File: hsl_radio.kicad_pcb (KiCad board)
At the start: 4 copper layers, 95.9 x 90.2 mm, 77 parts, among them J2 CC Prog/Debug, J4 UART1, J5 Control Outputs, J6 ANT, U1 AP62300TWU-7, U10 SKY65366-21, U2 CC1110, U3 SF2446E, U4 PCI-104, U5 TLV803S, U6 PE4259, U7 0433BM15A0001, U8 FT5HN 27MHz

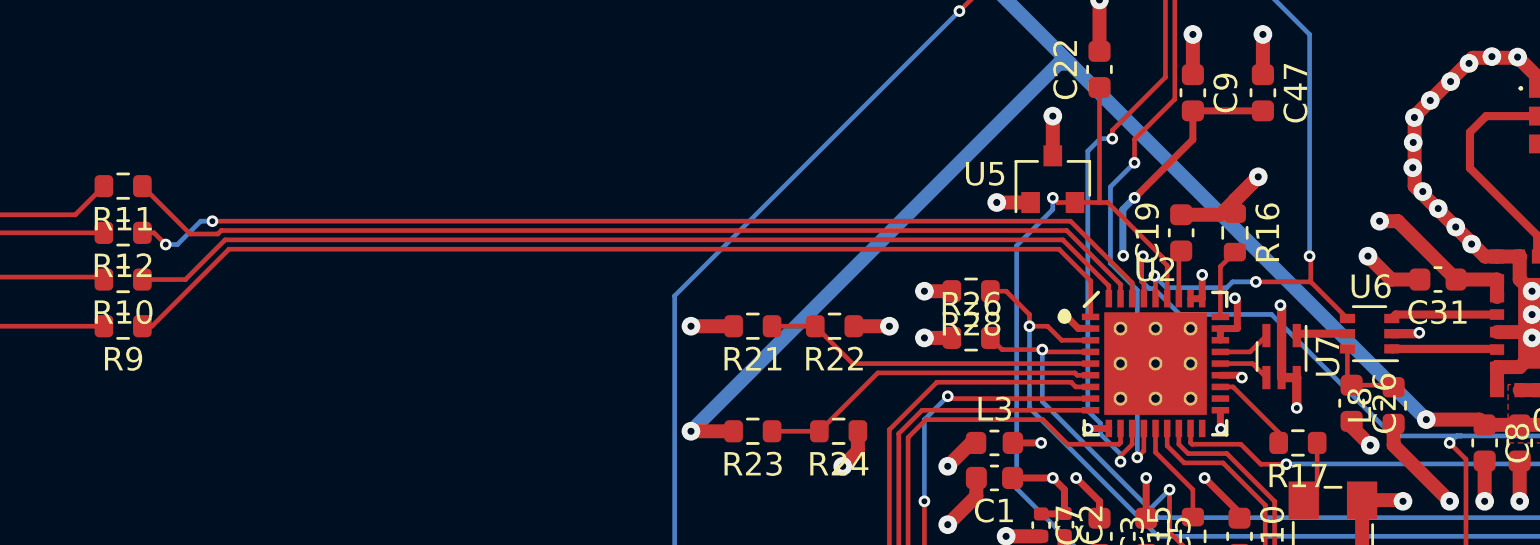
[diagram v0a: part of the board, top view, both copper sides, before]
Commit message: Finalized things
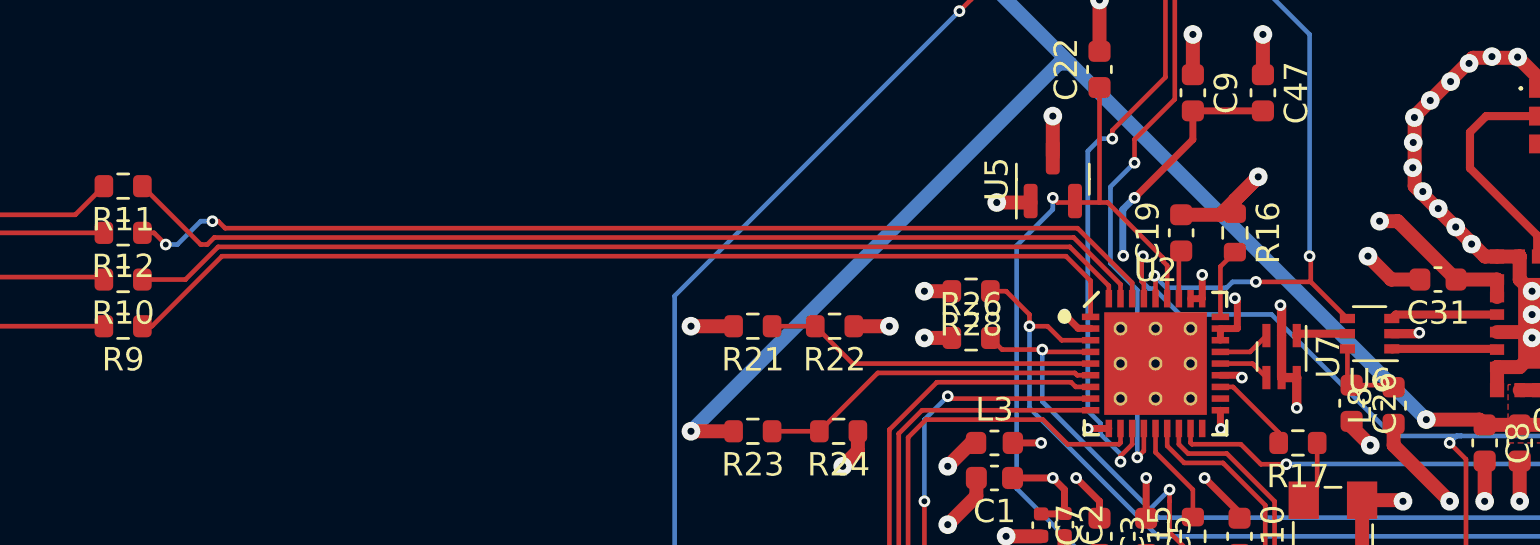
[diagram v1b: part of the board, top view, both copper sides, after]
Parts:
- U5: footprint archive:SOT-23 -> Package_TO_SOT_SMD:SOT-23
- U6: footprint archive:SOT-363_SC-70-6 -> Package_TO_SOT_SMD:SOT-363_SC-70-6
